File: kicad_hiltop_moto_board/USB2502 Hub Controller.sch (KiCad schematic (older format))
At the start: 49 parts, among them U27 USB2502, U7 DNF, Y1 50ppm 24.000MHZ

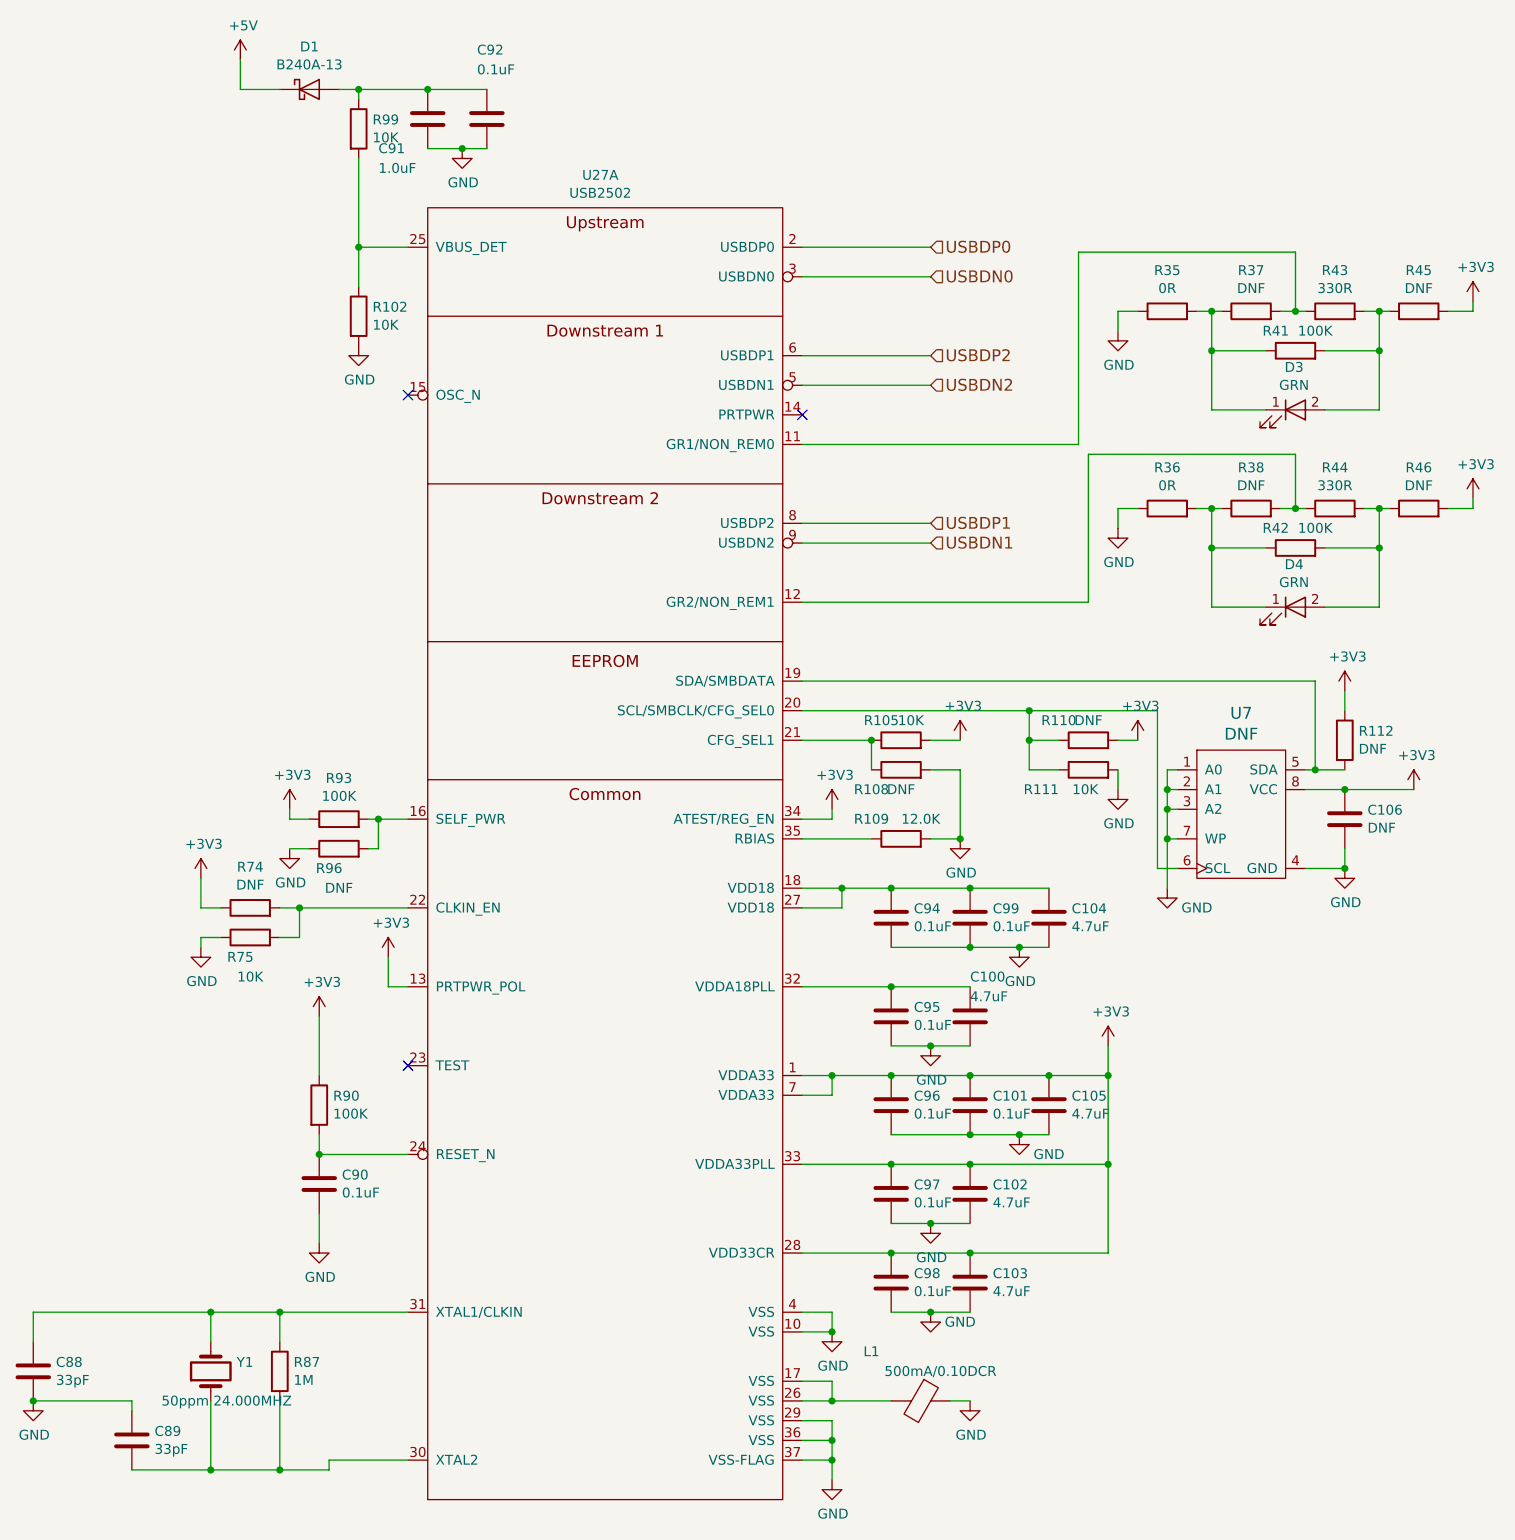
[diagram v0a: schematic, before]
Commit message: Moto board awaiting review
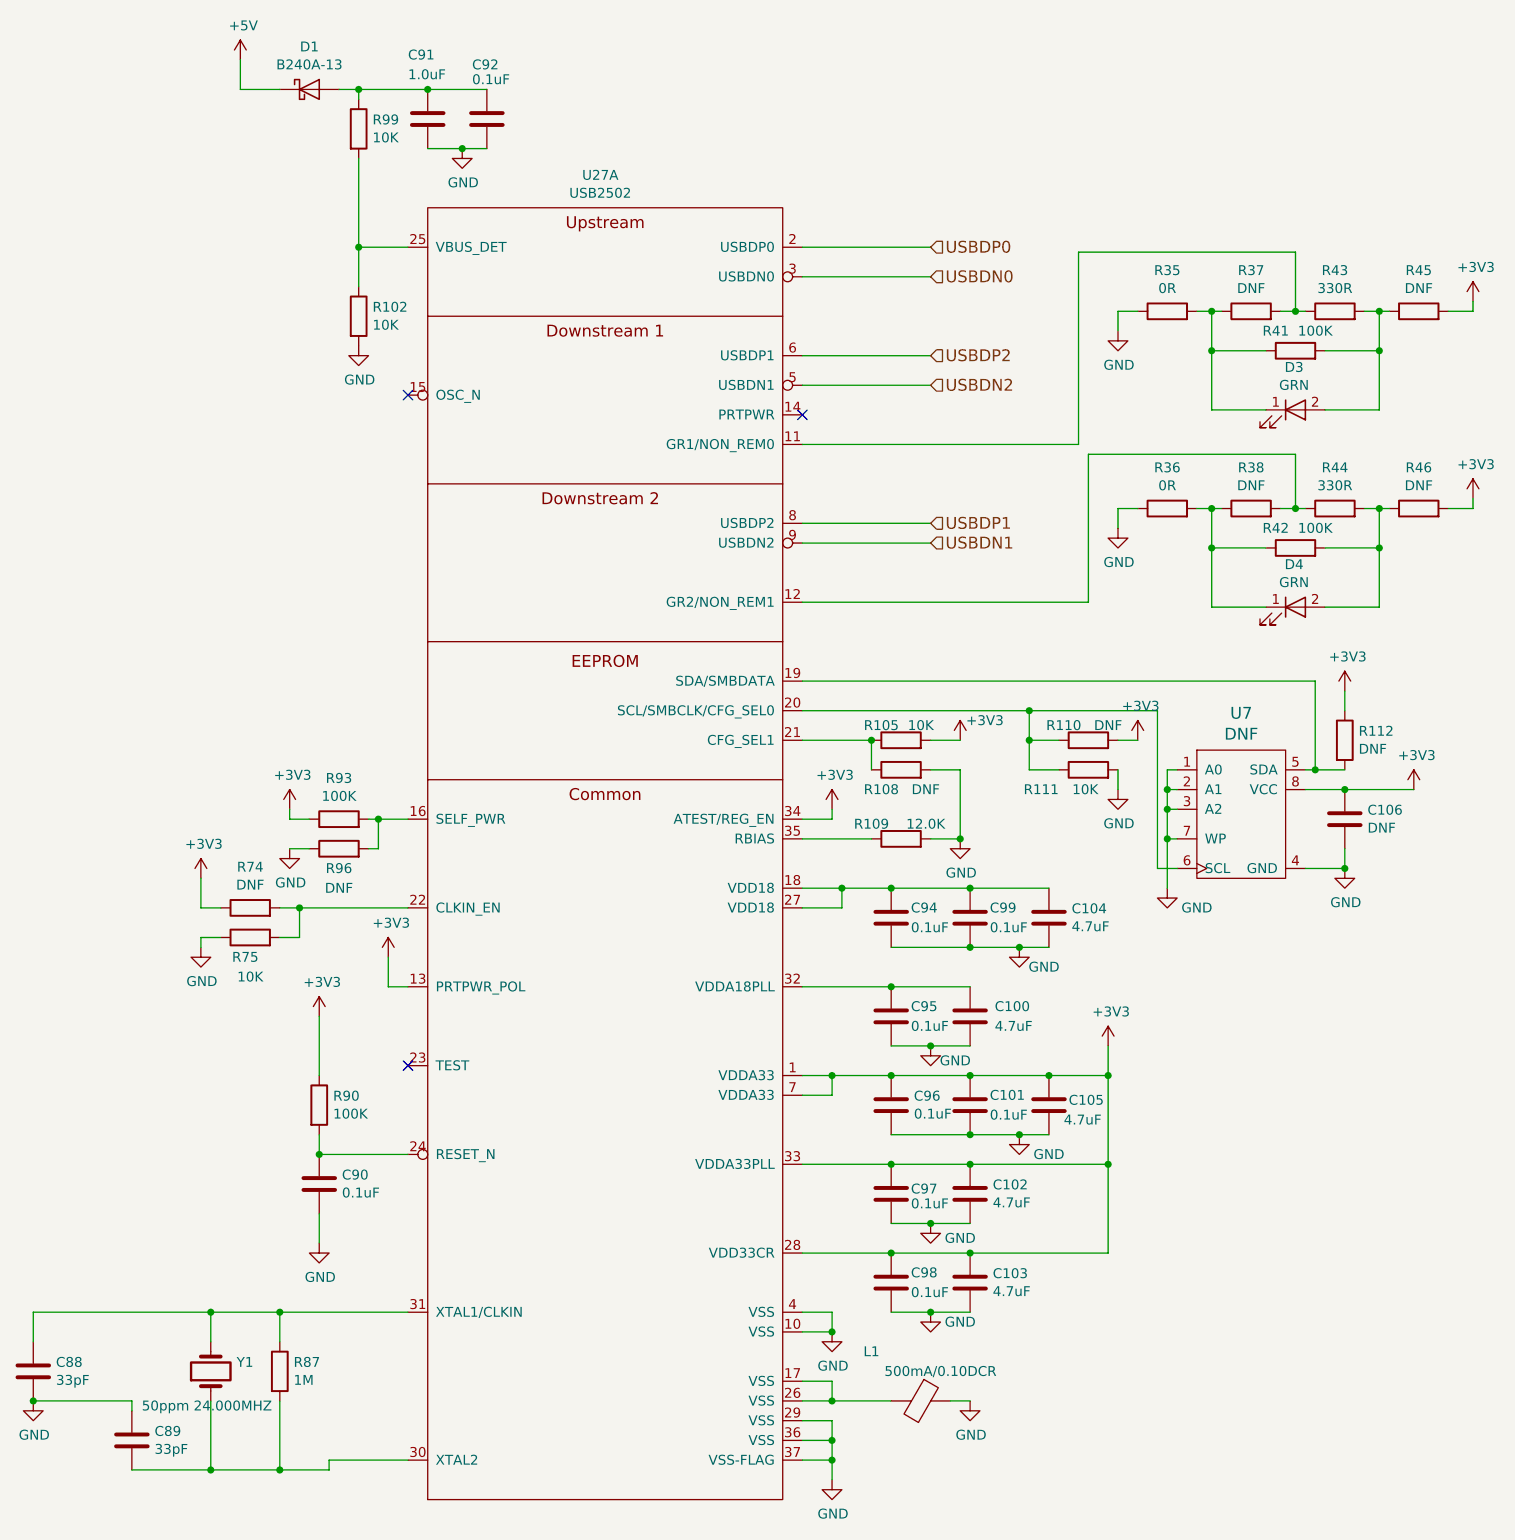
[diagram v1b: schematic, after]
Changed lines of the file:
@@
 P 4150 8550
 F 0 "Y1" V 4196 8419 50  0000 R CNN
-F 1 "50ppm 24.000MHZ" V 4000 8800 50  0000 R CNN
+F 1 "50ppm 24.000MHZ" V 3975 8900 50  0000 R CNN
 F 2 "Crystal:Crystal_SMD_TXC_7A-2Pin_5x3.2mm" H 4150 8550 50  0001 C CNN
 F 3 "" H 4150 8550 50  0001 C CNN
@@
 U 1 1 5D8F3D03
 P 7650 5500
-F 0 "R108" V 7550 5650 50  0000 C CNN
-F 1 "DNF" V 7550 5500 50  0000 C CNN
+F 0 "R108" V 7550 5600 50  0000 C CNN
+F 1 "DNF" V 7550 5375 50  0000 C CNN
 F 2 "Resistor_SMD:R_0603_1608Metric" V 7580 5500 50  0001 C CNN
 F 3 "" H 7650 5500 50  0001 C CNN
@@
 U 1 1 5D909BDF
 P 8000 7200
-F 0 "C101" H 8115 7246 50  0000 L CNN
-F 1 "0.1uF" H 8115 7155 50  0000 L CNN
+F 0 "C101" H 8100 7250 50  0000 L CNN
+F 1 "0.1uF" H 8100 7150 50  0000 L CNN
 F 2 "Capacitor_SMD:C_0402_1005Metric" H 8038 7050 50  0001 C CNN
 F 3 "" H 8000 7200 50  0001 C CNN
@@
 U 1 1 5D909BE5
 P 8400 7200
-F 0 "C105" H 8515 7246 50  0000 L CNN
-F 1 "4.7uF " H 8515 7155 50  0000 L CNN
+F 0 "C105" H 8500 7225 50  0000 L CNN
+F 1 "4.7uF " H 8475 7125 50  0000 L CNN
 F 2 "Capacitor_SMD:C_0402_1005Metric" H 8438 7050 50  0001 C CNN
 F 3 "" H 8400 7200 50  0001 C CNN
@@
 U 1 1 5D919F57
 P 7600 7650
-F 0 "C97" H 7715 7696 50  0000 L CNN
-F 1 "0.1uF" H 7715 7605 50  0000 L CNN
+F 0 "C97" H 7700 7675 50  0000 L CNN
+F 1 "0.1uF" H 7700 7600 50  0000 L CNN
 F 2 "Capacitor_SMD:C_0402_1005Metric" H 7638 7500 50  0001 C CNN
 F 3 "" H 7600 7650 50  0001 C CNN
@@
 U 1 1 5D929924
 P 7600 6750
-F 0 "C95" H 7715 6796 50  0000 L CNN
-F 1 "0.1uF" H 7715 6705 50  0000 L CNN
+F 0 "C95" H 7700 6800 50  0000 L CNN
+F 1 "0.1uF" H 7700 6700 50  0000 L CNN
 F 2 "Capacitor_SMD:C_0402_1005Metric" H 7638 6600 50  0001 C CNN
 F 3 "" H 7600 6750 50  0001 C CNN
@@
 U 1 1 5D92992A
 P 8000 6750
-F 0 "C100" H 8000 6950 50  0000 L CNN
-F 1 "4.7uF " H 8000 6850 50  0000 L CNN
+F 0 "C100" H 8125 6800 50  0000 L CNN
+F 1 "4.7uF " H 8125 6700 50  0000 L CNN
 F 2 "Capacitor_SMD:C_0402_1005Metric" H 8038 6600 50  0001 C CNN
 F 3 "" H 8000 6750 50  0001 C CNN
@@
 U 1 1 5D938ADF
 P 8000 6250
-F 0 "C99" H 8115 6296 50  0000 L CNN
-F 1 "0.1uF" H 8115 6205 50  0000 L CNN
+F 0 "C99" H 8100 6300 50  0000 L CNN
+F 1 "0.1uF" H 8100 6200 50  0000 L CNN
 F 2 "Capacitor_SMD:C_0402_1005Metric" H 8038 6100 50  0001 C CNN
 F 3 "" H 8000 6250 50  0001 C CNN
@@
 U 1 1 5D938AEB
 P 7600 6250
-F 0 "C94" H 7715 6296 50  0000 L CNN
-F 1 "0.1uF" H 7715 6205 50  0000 L CNN
+F 0 "C94" H 7700 6300 50  0000 L CNN
+F 1 "0.1uF" H 7700 6200 50  0000 L CNN
 F 2 "Capacitor_SMD:C_0402_1005Metric" H 7638 6100 50  0001 C CNN
 F 3 "" H 7600 6250 50  0001 C CNN
@@
 U 1 1 5D947DA8
 P 7650 5350
-F 0 "R105" V 7750 5450 50  0000 C CNN
-F 1 "10K" V 7750 5300 50  0000 C CNN
+F 0 "R105" V 7725 5450 50  0000 C CNN
+F 1 "10K" V 7725 5250 50  0000 C CNN
 F 2 "Resistor_SMD:R_0603_1608Metric" V 7580 5350 50  0001 C CNN
 F 3 "" H 7650 5350 50  0001 C CNN
@@
 U 1 1 5D949CAE
 P 8600 5350
-F 0 "R110" V 8700 5500 50  0000 C CNN
-F 1 "DNF" V 8700 5350 50  0000 C CNN
+F 0 "R110" V 8675 5475 50  0000 C CNN
+F 1 "DNF" V 8675 5250 50  0000 C CNN
 F 2 "Resistor_SMD:R_0603_1608Metric" V 8530 5350 50  0001 C CNN
 F 3 "" H 8600 5350 50  0001 C CNN
@@
 P 8250 6400
 F 0 "#PWR0208" H 8250 6150 50  0001 C CNN
-F 1 "GND" H 8255 6227 50  0000 C CNN
+F 1 "GND" H 8375 6300 50  0000 C CNN
 F 2 "" H 8250 6400 50  0001 C CNN
 F 3 "" H 8250 6400 50  0001 C CNN
@@
 U 1 1 5D9DC3FF
 P 4350 6350
-F 0 "R75" V 4250 6400 50  0000 C CNN
+F 0 "R75" V 4250 6375 50  0000 C CNN
 F 1 "10K " V 4150 6350 50  0000 C CNN
 F 2 "Resistor_SMD:R_0603_1608Metric" V 4280 6350 50  0001 C CNN
@@
 U 1 1 5D9E4A4E
 P 4800 5900
-F 0 "R96" V 4700 5950 50  0000 C CNN
+F 0 "R96" V 4700 5900 50  0000 C CNN
 F 1 "DNF" V 4600 5900 50  0000 C CNN
 F 2 "Resistor_SMD:R_0603_1608Metric" V 4730 5900 50  0001 C CNN
@@
 U 1 1 5D94B078
 P 7650 5850
-F 0 "R109" V 7750 6000 50  0000 C CNN
-F 1 "12.0K " V 7750 5750 50  0000 C CNN
+F 0 "R109" V 7725 6000 50  0000 C CNN
+F 1 "12.0K " V 7725 5725 50  0000 C CNN
 F 2 "Resistor_SMD:R_0603_1608Metric" V 7580 5850 50  0001 C CNN
 F 3 "" H 7650 5850 50  0001 C CNN
@@
 P 7800 6900
 F 0 "#PWR0217" H 7800 6650 50  0001 C CNN
-F 1 "GND" H 7805 6727 50  0000 C CNN
+F 1 "GND" H 7925 6825 50  0000 C CNN
 F 2 "" H 7800 6900 50  0001 C CNN
 F 3 "" H 7800 6900 50  0001 C CNN
@@
 P 7800 7800
 F 0 "#PWR0219" H 7800 7550 50  0001 C CNN
-F 1 "GND" H 7805 7627 50  0000 C CNN
+F 1 "GND" H 7950 7725 50  0000 C CNN
 F 2 "" H 7800 7800 50  0001 C CNN
 F 3 "" H 7800 7800 50  0001 C CNN
@@
 U 1 1 5D8FF0CE
 P 7600 8100
-F 0 "C98" H 7715 8146 50  0000 L CNN
-F 1 "0.1uF" H 7715 8055 50  0000 L CNN
+F 0 "C98" H 7700 8150 50  0000 L CNN
+F 1 "0.1uF" H 7700 8050 50  0000 L CNN
 F 2 "Capacitor_SMD:C_0402_1005Metric" H 7638 7950 50  0001 C CNN
 F 3 "" H 7600 8100 50  0001 C CNN
@@
 U 1 1 5DCA03F2
 P 5250 2200
-F 0 "C91" H 5000 2050 50  0000 L CNN
-F 1 "1.0uF " H 5000 1950 50  0000 L CNN
+F 0 "C91" H 5150 2525 50  0000 L CNN
+F 1 "1.0uF " H 5150 2425 50  0000 L CNN
 F 2 "Capacitor_SMD:C_0402_1005Metric" H 5288 2050 50  0001 C CNN
 F 3 "" H 5250 2200 50  0001 C CNN
@@
 U 1 1 5DCA2D03
 P 5550 2200
-F 0 "C92" H 5500 2550 50  0000 L CNN
-F 1 "0.1uF" H 5500 2450 50  0000 L CNN
+F 0 "C92" H 5475 2475 50  0000 L CNN
+F 1 "0.1uF" H 5475 2400 50  0000 L CNN
 F 2 "Capacitor_SMD:C_0402_1005Metric" H 5588 2050 50  0001 C CNN
 F 3 "" H 5550 2200 50  0001 C CNN
@@
 AR Path="/5D8D08E6/5E674F93" Ref="#PWR0202"  Part="1"
 F 0 "#PWR0202" H 7950 5200 50  0001 C CNN
-F 1 "+3V3" H 7965 5523 50  0000 C CNN
+F 1 "+3V3" H 8075 5450 50  0000 C CNN
 F 2 "" H 7950 5350 50  0001 C CNN
 F 3 "" H 7950 5350 50  0001 C CNN
